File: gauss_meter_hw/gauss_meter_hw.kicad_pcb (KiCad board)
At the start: 2 copper layers, 15 parts, among them J1 Conn_01x04, U1 INA326

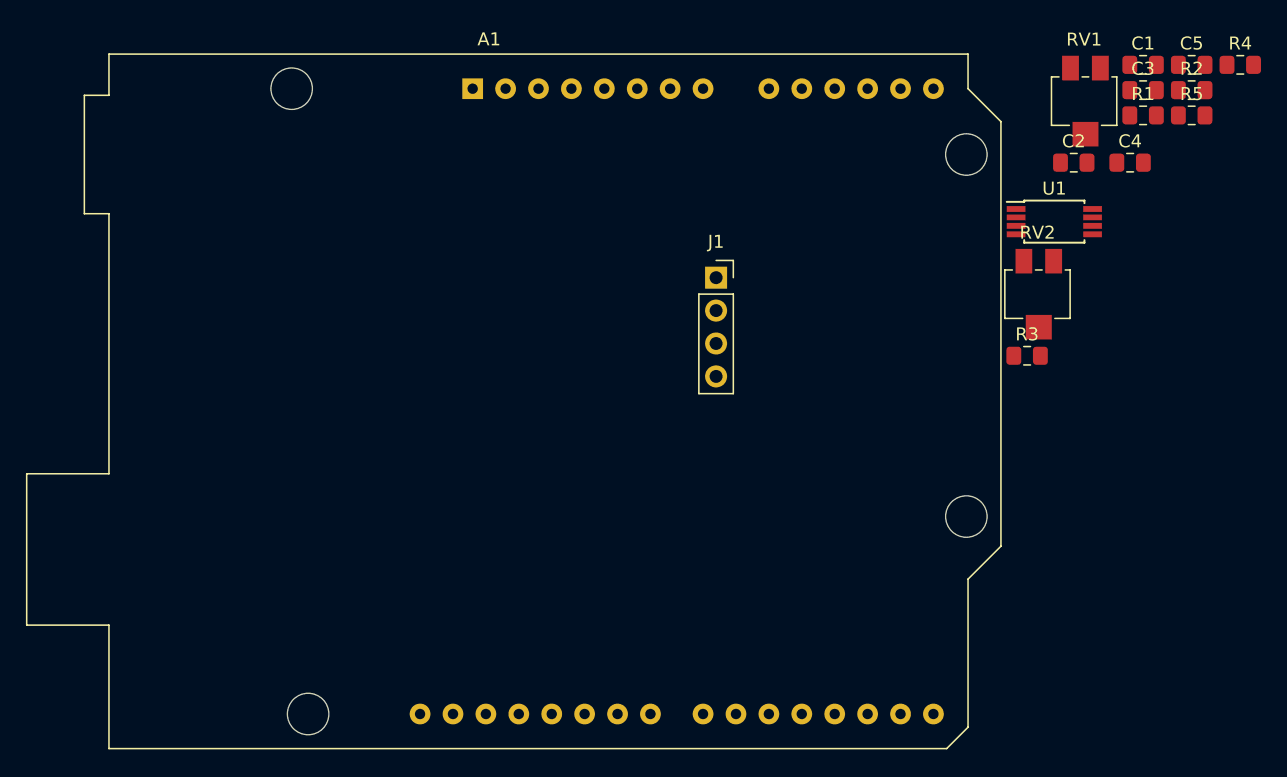
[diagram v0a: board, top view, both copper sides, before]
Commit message: initial PCB design
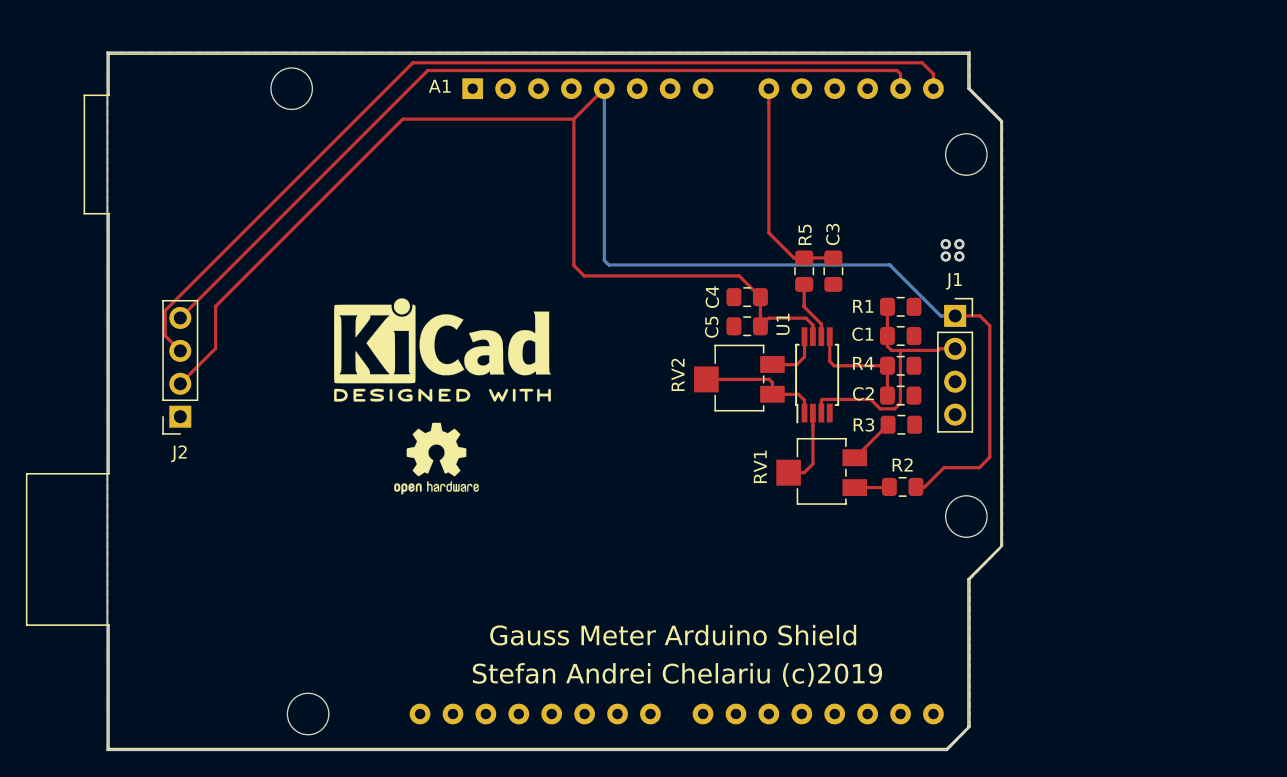
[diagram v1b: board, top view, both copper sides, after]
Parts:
- added J2: 128x64 - SSH1106, Connector_PinSocket_2.54mm:PinSocket_1x04_P2.54mm_Vertical, F.Cu at (121.7, 89.3)
- added REF**: KiCad-Logo2_8mm_SilkScreen, Symbol:KiCad-Logo2_8mm_SilkScreen, F.Cu at (141.9, 84.1)
- added REF**: OSHW-Logo2_7.3x6mm_SilkScreen, Symbol:OSHW-Logo2_7.3x6mm_SilkScreen, F.Cu at (141.5, 92.5)
- moved C5 39.8 mm to (165.4, 82.3), turned to 180 degrees
- moved R2 37.9 mm to (177.4, 94.7)
- moved RV1 35.2 mm to (171.2, 93.6), turned to 270 degrees
- moved R4 35.0 mm to (177.3, 85.3)
- moved R5 32.2 mm to (169.8, 78.0), turned to 270 degrees
- moved C4 31.3 mm to (165.4, 80.0), turned to 180 degrees
- moved C1 28.1 mm to (177.3, 83.0)
- moved C3 27.7 mm to (172.1, 78.0), turned to 270 degrees
- moved RV2 24.0 mm to (164.8, 86.4), turned to 270 degrees
- moved R1 23.8 mm to (177.3, 80.8)
- moved C2 22.4 mm to (177.3, 87.7)
- moved U1 21.8 mm to (170.8, 86.0), turned to 90 degrees
- moved J1 18.7 mm to (181.5, 81.5)
- moved R3 11.1 mm to (177.3, 89.9), turned to 180 degrees
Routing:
- net +5V: track 0.00 -> 140.3 mm
- net Net-(A1-Pad14): track 0.00 -> 72.3 mm
- net Net-(A1-Pad13): track 0.00 -> 64.7 mm
- net Net-(C1-Pad1): track 0.00 -> 20.1 mm
- net Net-(A1-Pad9): track 0.00 -> 16.9 mm
- net Net-(RV2-Pad1): track 0.00 -> 9.76 mm
- net Net-(C2-Pad1): track 0.00 -> 8.80 mm
- net Net-(RV1-Pad2): track 0.00 -> 6.08 mm
- net Net-(R5-Pad2): track 0.00 -> 4.59 mm
- net Net-(RV2-Pad3): track 0.00 -> 4.29 mm
- net Net-(R3-Pad2): track 0.00 -> 3.63 mm
- net Net-(R2-Pad1): track 0.00 -> 2.70 mm
- net GND: vias 0 -> 4
- added copper zone on B.Cu, net GND
- added copper zone on F.Cu, net GND
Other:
- board outline added: 69 x 53.9 mm
- board text added: "Gauss Meter Arduino Shield"
- board text added: "Stefan Andrei Chelariu (c)2019"
